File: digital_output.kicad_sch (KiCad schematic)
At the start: 12 parts, among them Q1 AOSP21321, Q2 AOSP21321, Q3 NMOS, Q4 NMOS

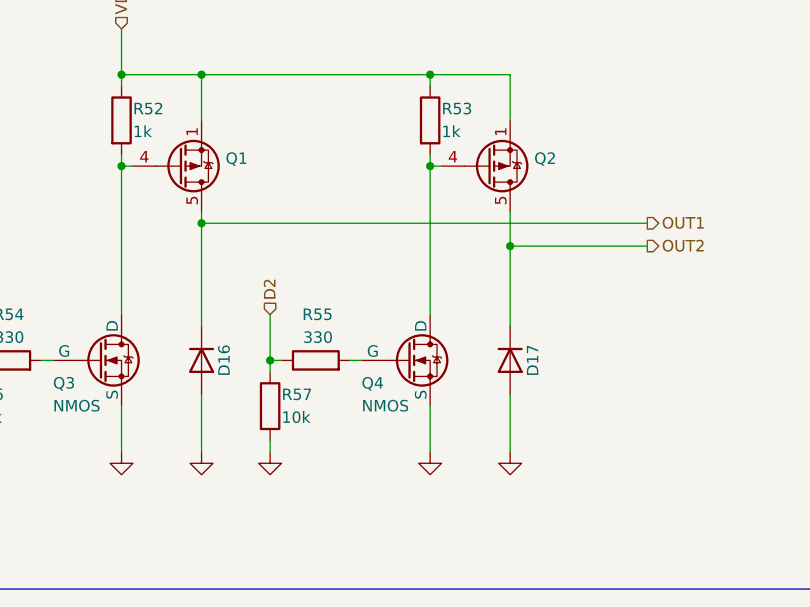
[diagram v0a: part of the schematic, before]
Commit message: more routing
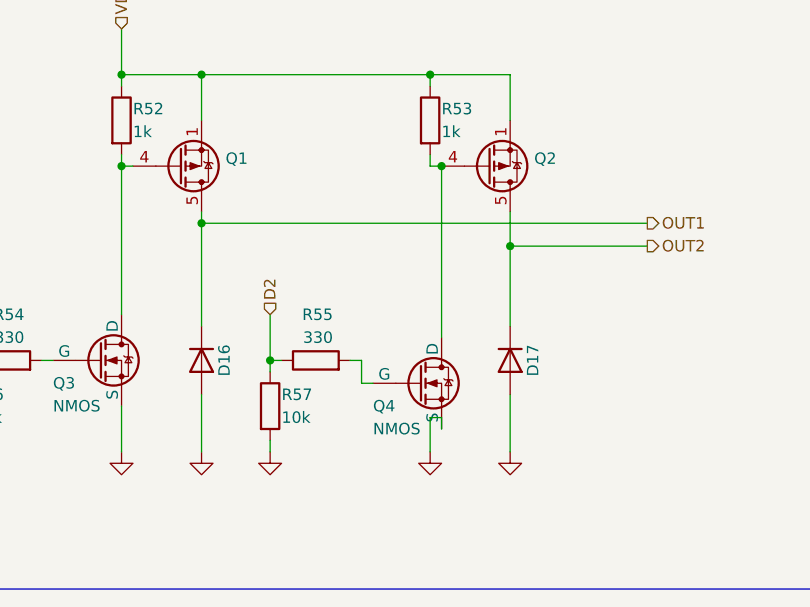
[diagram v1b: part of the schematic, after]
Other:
- moved on the sheet: Q4
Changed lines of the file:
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@@
+	)
+	(junction
+		(at 72.39 67.31)
+		(diameter 0)
+		(color 0 0 0 0)
 	)
 	(junction
@@
 		(color 0 0 0 0)
 	)
-	(junction
-		(at 71.12 67.31)
-		(diameter 0)
-		(color 0 0 0 0)
-	)
 	(wire
 		(pts
@@
 	(wire
 		(pts
+			(xy 63.5 88.9) (xy 62.23 88.9)
+		)
+		(stroke
+			(width 0)
+			(type default)
+		)
+	)
+	(wire
+		(pts
 			(xy 36.83 58.42) (xy 36.83 57.15)
 		)
@@
 	(wire
 		(pts
+			(xy 72.39 67.31) (xy 71.12 67.31)
+		)
+		(stroke
+			(width 0)
+			(type default)
+		)
+	)
+	(wire
+		(pts
+			(xy 63.5 91.44) (xy 63.5 88.9)
+		)
+		(stroke
+			(width 0)
+			(type default)
+		)
+	)
+	(wire
+		(pts
 			(xy 19.05 83.82) (xy 19.05 88.9)
 		)
@@
 	(wire
 		(pts
-			(xy 71.12 67.31) (xy 71.12 83.82)
+			(xy 72.39 67.31) (xy 72.39 86.36)
 		)
 		(stroke
@@
 	(wire
 		(pts
+			(xy 71.12 95.25) (xy 71.12 99.06)
+		)
+		(stroke
+			(width 0)
+			(type default)
+		)
+	)
+	(wire
+		(pts
 			(xy 53.34 83.82) (xy 53.34 88.9)
 		)
@@
 	(wire
 		(pts
-			(xy 71.12 93.98) (xy 71.12 99.06)
+			(xy 72.39 96.52) (xy 72.39 95.25)
 		)
 		(stroke
@@
 	(wire
 		(pts
-			(xy 71.12 67.31) (xy 72.39 67.31)
-		)
-		(stroke
-			(width 0)
-			(type default)
-		)
-	)
-	(wire
-		(pts
 			(xy 53.34 90.17) (xy 53.34 88.9)
 		)
@@
 	(wire
 		(pts
-			(xy 62.23 88.9) (xy 63.5 88.9)
+			(xy 63.5 91.44) (xy 64.77 91.44)
 		)
 		(stroke
@@
 		(pts
 			(xy 27.94 88.9) (xy 29.21 88.9)
+		)
+		(stroke
+			(width 0)
+			(type default)
+		)
+	)
+	(wire
+		(pts
+			(xy 72.39 95.25) (xy 71.12 95.25)
 		)
 		(stroke
@@
 	(symbol
 		(lib_id "Simulation_SPICE:NMOS")
-		(at 68.58 88.9 0)
+		(at 69.85 91.44 0)
 		(unit 1)
 		(exclude_from_sim no)
@@
 		(dnp no)
 		(property "Reference" "Q4"
-			(at 63.5 91.44 0)
+			(at 64.77 93.98 0)
 			(effects
 				(font
@@
 		)
 		(property "Value" "NMOS"
-			(at 63.5 93.98 0)
+			(at 64.77 96.52 0)
 			(effects
 				(font
@@
 		)
 		(property "Footprint" "Package_TO_SOT_SMD:SOT-23"
-			(at 73.66 86.36 0)
+			(at 74.93 88.9 0)
 			(effects
 				(font
@@
 		)
 		(property "Datasheet" "https://ngspice.sourceforge.io/docs/ngspice-manual.pdf"
-			(at 68.58 101.6 0)
+			(at 69.85 104.14 0)
 			(effects
 				(font
@@
 		)
 		(property "Description" ""
-			(at 68.58 88.9 0)
+			(at 69.85 91.44 0)
 			(effects
 				(font
@@
 		)
 		(property "Sim.Device" "NMOS"
-			(at 68.58 106.045 0)
+			(at 69.85 108.585 0)
 			(effects
 				(font
@@
 		)
 		(property "Sim.Type" "VDMOS"
-			(at 68.58 107.95 0)
+			(at 69.85 110.49 0)
 			(effects
 				(font
@@
 		)
 		(property "Sim.Pins" "1=D 2=G 3=S"
-			(at 68.58 104.14 0)
+			(at 69.85 106.68 0)
 			(effects
 				(font
@@
 		)
 		(property "LCSC#" "C20917"
-			(at 68.58 88.9 0)
+			(at 69.85 91.44 0)
 			(effects
 				(font
@@
 		)
 		(property "Manufacturer" "Alpha & Omega Semicon"
-			(at 68.58 88.9 0)
+			(at 69.85 91.44 0)
 			(effects
 				(font
@@
 		)
 		(property "Part#" "AO3400A"
-			(at 68.58 88.9 0)
-			(effects
-				(font
+			(at 69.85 91.44 0)
+			(effects
+				(font
